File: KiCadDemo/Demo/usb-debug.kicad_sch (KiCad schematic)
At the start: 3 parts, among them J7 USB_B_Mini, J8 Debug

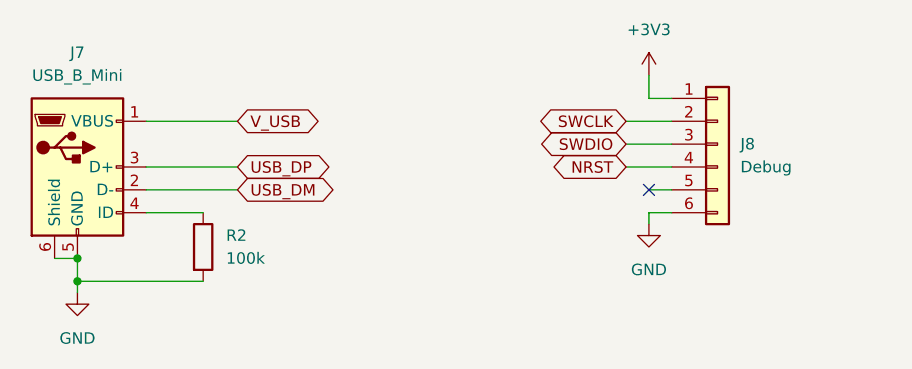
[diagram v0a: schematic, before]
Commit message: Add files via upload
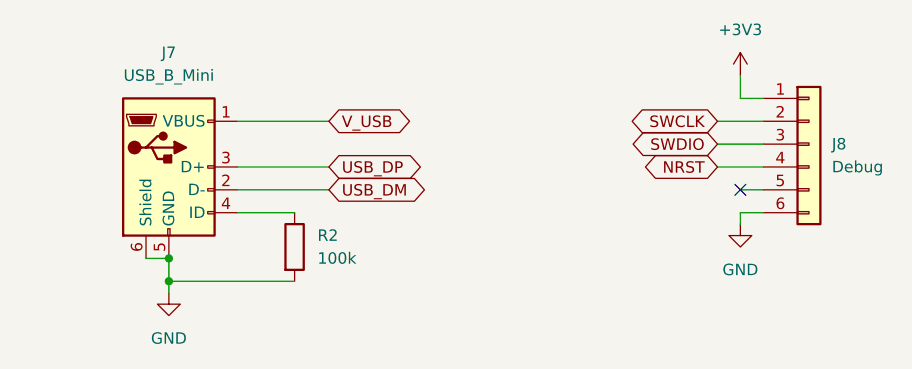
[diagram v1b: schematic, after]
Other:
- moved on the sheet: J7, J8, R2

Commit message: Check #4
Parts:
- J8: footprint (none) -> Demo:Debug
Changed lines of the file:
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@@
       (effects (font (size 1.27 1.27)) (justify left))
     )
-    (property "Footprint" "" (at 182.88 85.09 0)
+    (property "Footprint" "Demo:Debug" (at 182.88 85.09 0)
       (effects (font (size 1.27 1.27)) hide)
     )
